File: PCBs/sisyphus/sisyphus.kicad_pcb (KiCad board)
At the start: 2 copper layers, 52 x 42 mm, 69 parts, among them J1 Light sensor, J10 Keyboard, J2 USB_C_Receptacle_USB2.0_14P, J3 AUX USB, J4 USB_BOOT, J5 Speaker, J6 Battery, J7 SWD, J8 Limit SW, J9 RGB_CONN, Q1 AO3401A, SW1 SW_SPDT_321, U1 TPS62293, U2 USBLC6-2P6, U3 BQ25619, U4 W25Q128JVS, U5 MAX98357A, U7 RP2040, U8 TCA8418, Y1 ABM8-272-T3

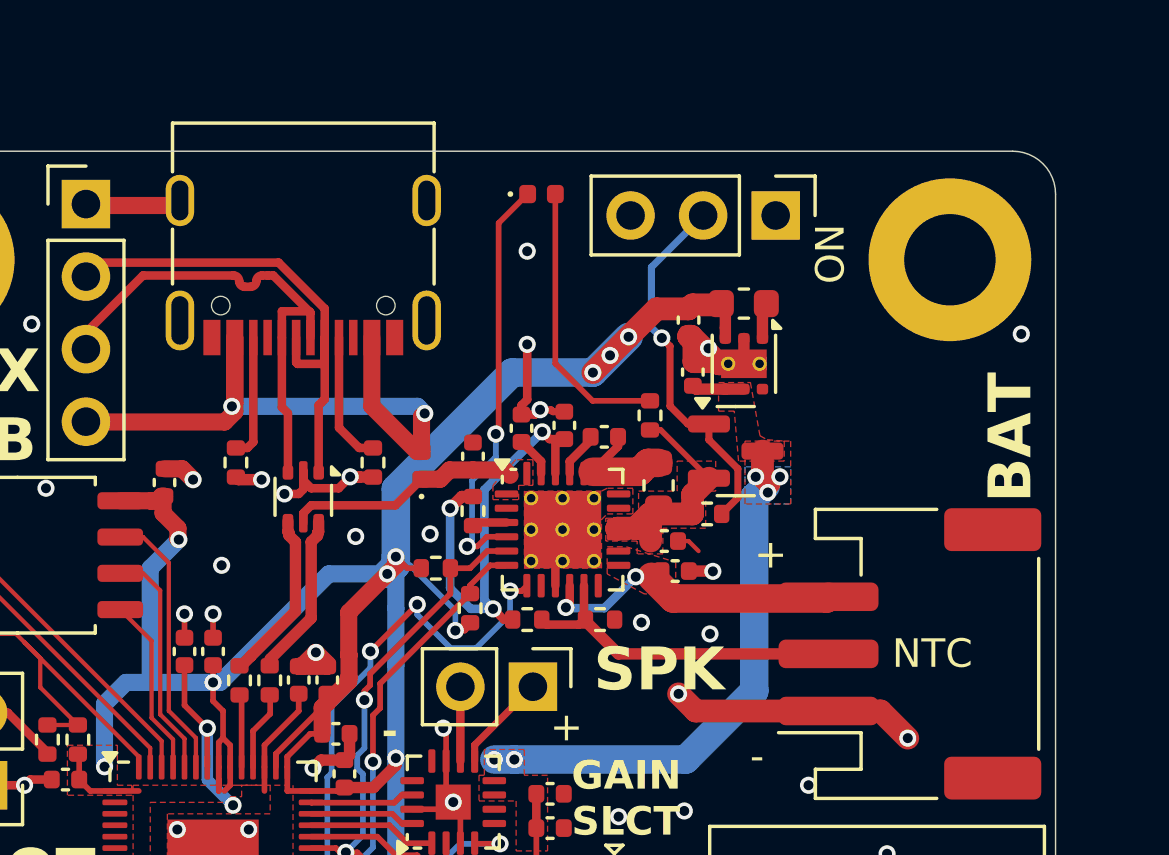
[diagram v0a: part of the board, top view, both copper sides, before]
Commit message: Add the first actually ordered version of the PCB
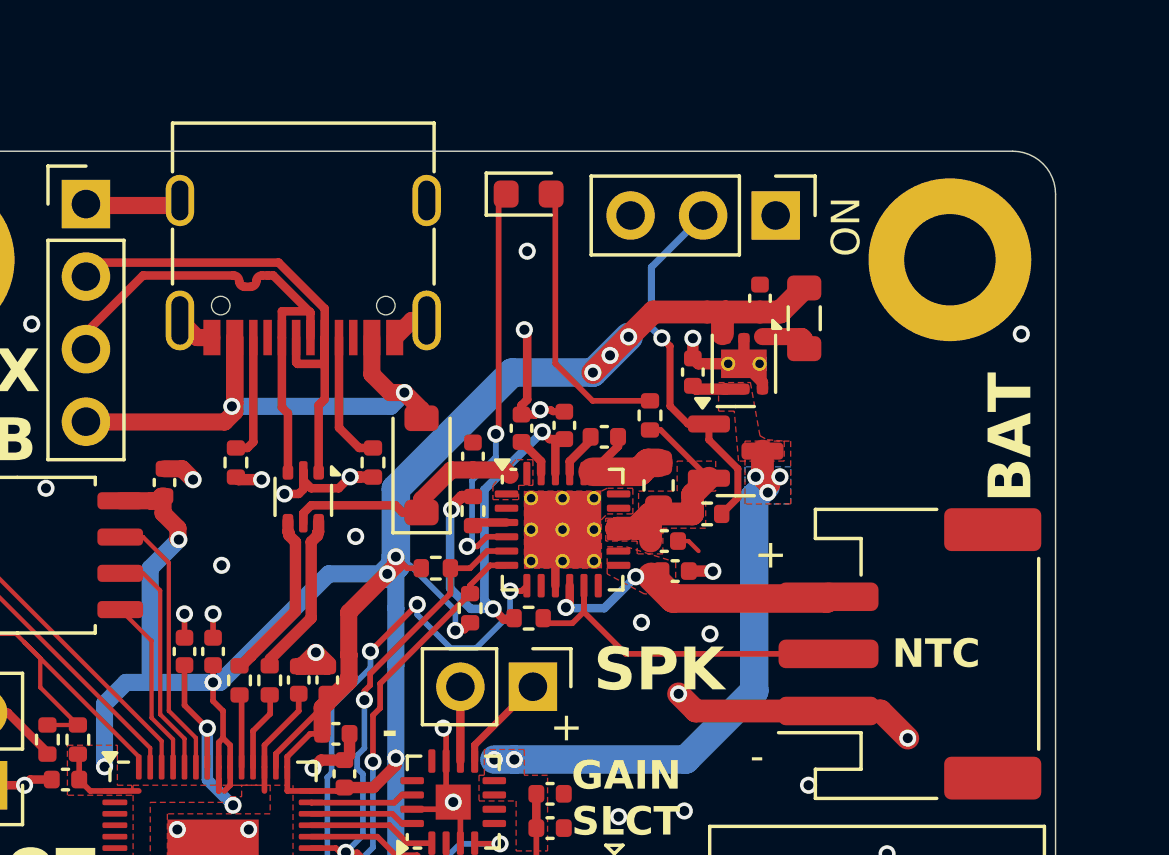
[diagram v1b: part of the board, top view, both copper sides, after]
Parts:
- removed the R6 at (111.0, 91.4)
- removed the R7 at (113.5, 91.4)
- added R11: 10k, Resistor_SMD:R_0402_1005Metric, F.Cu at (111.0, 91.3)
- D1: renamed from D2; footprint LED_SMD:LED_0402_1005Metric -> LED_SMD:LED_0603_1608Metric
- D2: renamed from D1; value D_Schottky -> D_shottky; footprint Diode_SMD:D_0402_1005Metric -> Diode_SMD:D_SOD-123
- L2: footprint Inductor_SMD:L_0603_1608Metric -> Inductor_SMD:L_0805_2012Metric
- R3: renamed from R11; value 27 -> 33
- R4: renamed from R12; value 27 -> 33
- R9: renamed from R4; value 220 -> 330
- U3: renamed from U1; value TPS62293 -> TPS62291
- moved C20 2.62 mm to (119.2, 80.2), turned to 90 degrees
- moved L2 2.18 mm to (120.7, 80.8), turned to -90 degrees
- moved D1 0.45 mm to (111.0, 76.5)
- renumbered C20 to C1, C13 to C10, C22 to C11, C21 to C12, C26 to C13, C23 to C14, C24 to C15, C1 to C16, C2 to C17, C3 to C18, C4 to C19, C19 to C2, C5 to C20, C6 to C21, C7 to C22, C8 to C23, C9 to C24, C10 to C25, C18 to C3, C17 to C4, C16 to C5, C15 to C6, C14 to C7, C11 to C8, C12 to C9, H4 to H1, H3 to H2, H2 to H3, H1 to H4, J4 to J1, J5 to J10, J7 to J2, J6 to J3, J2 to J4, J10 to J5, J3 to J6, J1 to J7, R8 to R1, R5 to R10, R2 to R12, R3 to R13, R10 to R14, R9 to R2, R13 to R5, R14 to R6, R15 to R7, R1 to R8, U4 to U1, U7 to U2, U3 to U4, U2 to U5, U8 to U6, U5 to U7
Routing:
- net VBUS: track 23.4 -> 20.5 mm
- net +3V3: track 130.4 -> 133.1 mm
- net GND: track 55.3 -> 57.2 mm, vias 62 -> 61
- net /Batery and power/NTC: track 11.9 -> 12.7 mm
- net Net-(U3-SW): track 1.23 -> 1.84 mm
